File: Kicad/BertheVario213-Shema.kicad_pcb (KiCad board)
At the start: 2 copper layers, 8 parts

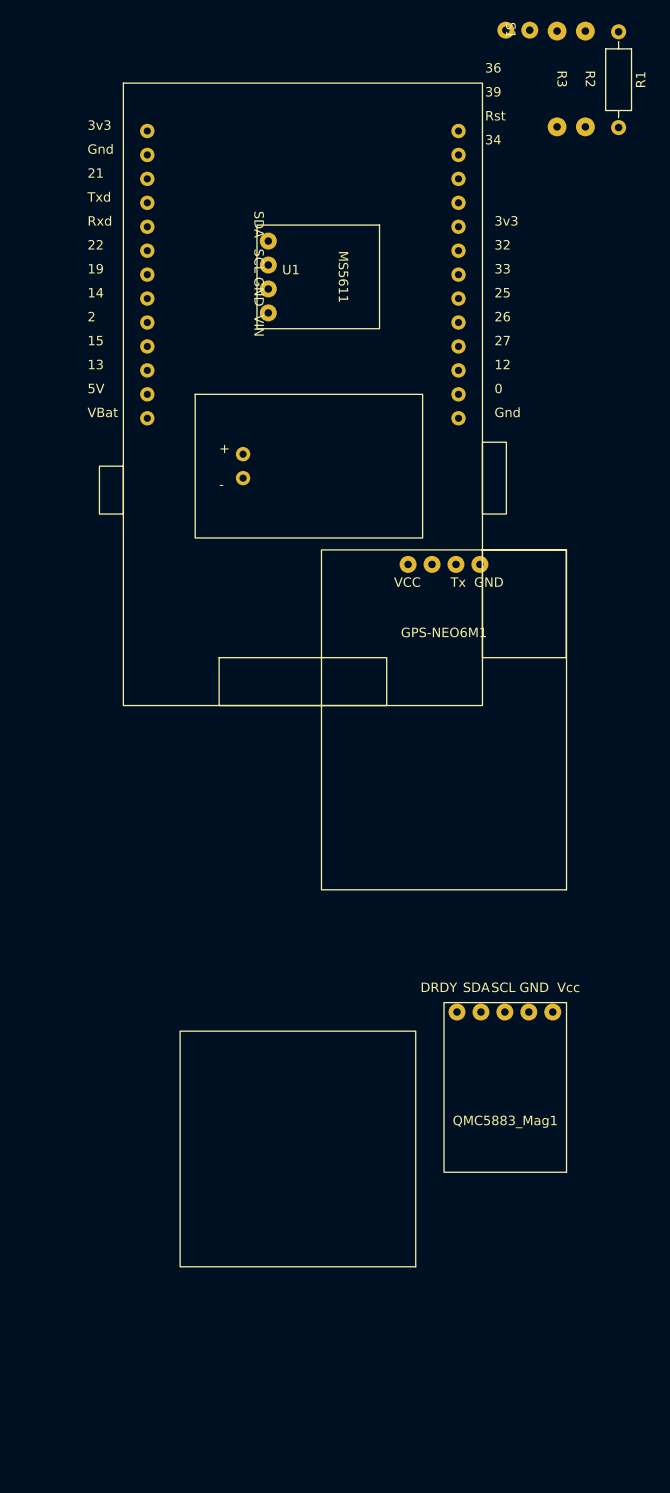
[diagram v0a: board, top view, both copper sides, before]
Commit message: progession pcb
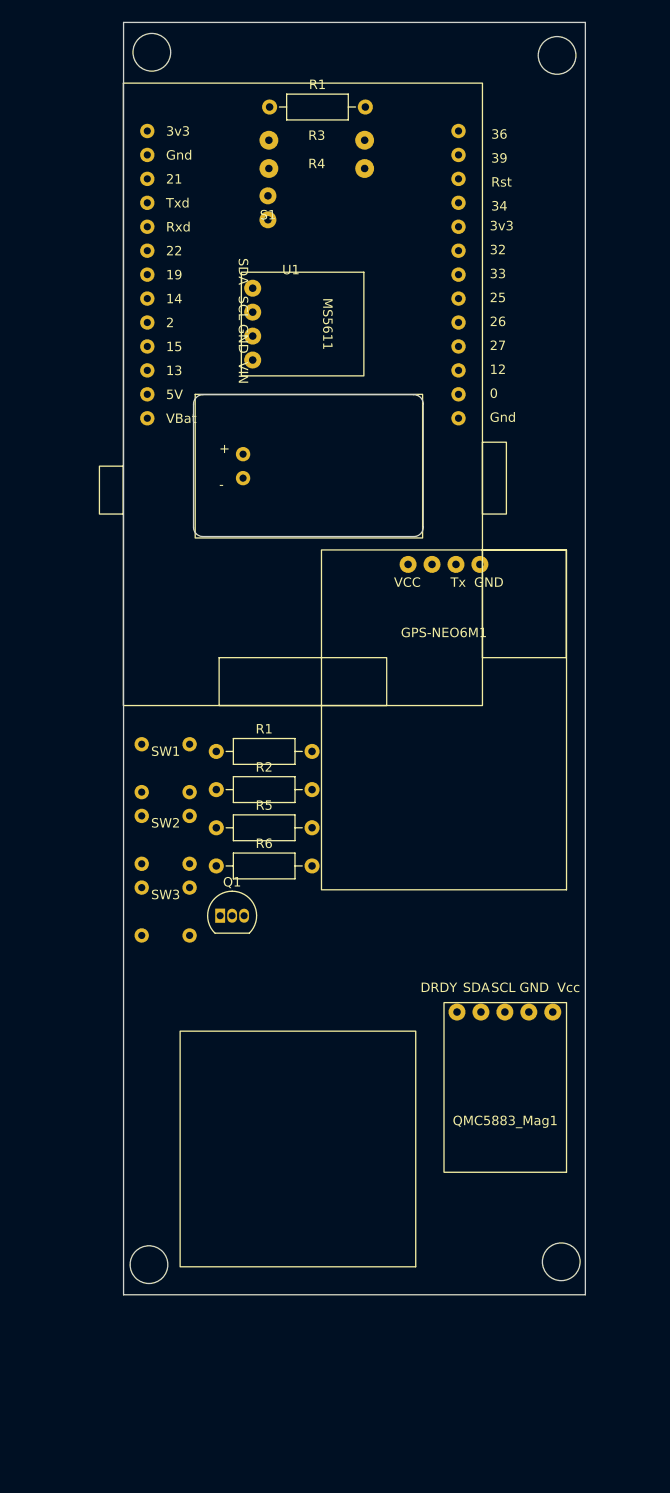
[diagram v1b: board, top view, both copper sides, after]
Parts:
- added Q1: S8050, Package_TO_SOT_THT:TO-92_Inline, F.Cu at (141.2, 117.3)
- added R1: 1K, Resistor_THT:R_Axial_DIN0207_L6.3mm_D2.5mm_P10.16mm_Horizontal, F.Cu at (140.8, 99.8)
- added R2: 10k, Resistor_THT:R_Axial_DIN0207_L6.3mm_D2.5mm_P10.16mm_Horizontal, F.Cu at (140.8, 103.9)
- added R5: 10K, Resistor_THT:R_Axial_DIN0207_L6.3mm_D2.5mm_P10.16mm_Horizontal, F.Cu at (140.8, 108.0)
- added R6: 10k, Resistor_THT:R_Axial_DIN0207_L6.3mm_D2.5mm_P10.16mm_Horizontal, F.Cu at (140.8, 112.0)
- added SW1: Gauche, BertheShema:switch, F.Cu at (135.5, 100.4)
- added SW2: Centre, BertheShema:switch, F.Cu at (135.5, 108.0)
- added SW3: Droit, BertheShema:switch, F.Cu at (135.5, 115.6)
- moved R1 37.9 mm to (146.5, 31.5), turned to 0 degrees
- moved S1 32.3 mm to (146.3, 43.4), turned to 0 degrees
- moved R3 29.2 mm to (151.5, 35.0), turned to 0 degrees
- moved R4 27.2 mm to (151.5, 38.0), turned to 0 degrees
- moved MS5611 5.27 mm to (147.1, 54.5)
- renumbered R2 to R3, R3 to R4
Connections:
- S1 pad 1: GNDREF -> Net-(Q1-C)
- S1 pad 2: Net-(R1-Pad1) -> Net-(U1-Vbat)
- U1 pad 13: (no net) -> Net-(U1-Bouton_Droit)
- U1 pad 14: (no net) -> Net-(U1-Bouton_Gauche)
- U1 pad 15: (no net) -> Net-(U1-Bouton_Centre)
- U1 pad 34: (no net) -> Net-(U1-Speaker)
- U1 pad 36: (no net) -> Net-(U1-VBat)
- U1 pad 6: unconnected-(U1-Vbat-Pad6) -> Net-(U1-Vbat)
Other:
- board outline added: 49 x 135 mm

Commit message: modif pcb
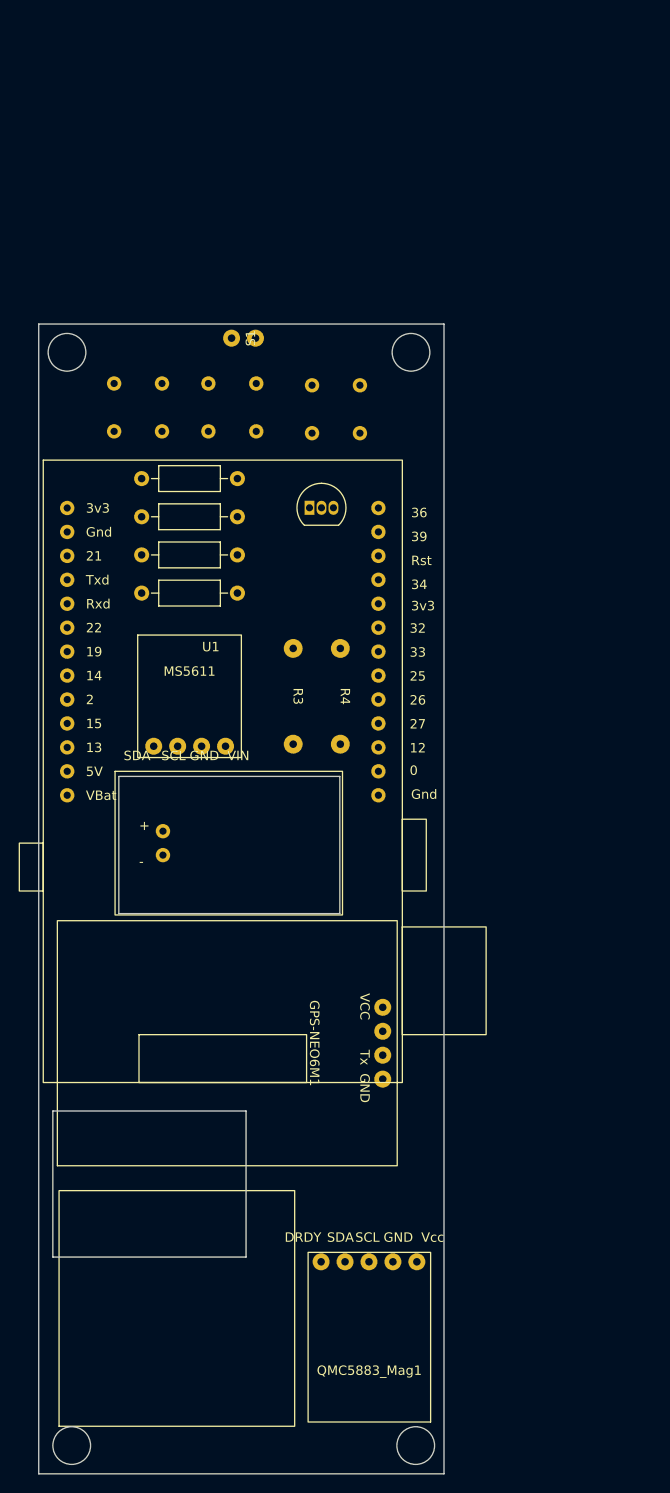
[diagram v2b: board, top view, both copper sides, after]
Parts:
- removed the R1 at (146.5, 31.5)
- S1: value Speaker 2W 8ohms -> Speaker 1W 80 ohms
- moved R3 59.1 mm to (149.0, 94.0), turned to -90 degrees
- moved R4 56.1 mm to (154.0, 94.0), turned to -90 degrees
- moved SW3 53.6 mm to (132.5, 62.1)
- moved GPS-NEO6M1 49.9 mm to (157.0, 130.8), turned to 90 degrees
- moved SW2 46.4 mm to (142.5, 62.1)
- moved Q1 44.3 mm to (150.7, 74.0)
- moved MS5611 43.4 mm to (138.0, 96.9), turned to 0 degrees
- moved SW1 42.2 mm to (153.5, 62.3)
- moved U1 40.9 mm to (140.3, 89.3)
- moved QMC5883_Mag1 30.2 mm to (157.1, 160.0)
- moved R2 30.0 mm to (132.9, 75.0)
- moved R5 30.0 mm to (132.9, 79.0)
- moved R6 30.0 mm to (132.9, 83.0)
- moved R1 30.0 mm to (132.9, 70.9)
- moved S1 12.6 mm to (145.0, 56.0), turned to 90 degrees
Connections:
- S1 pad 2: Net-(U1-Vbat) -> Net-(U1-5V)
- U1 pad 25: (no net) -> Net-(U1-Speaker)
- U1 pad 34: Net-(U1-Speaker) -> (no net)
- U1 pad 5: (no net) -> Net-(U1-5V)
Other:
- board size 49 x 135 mm -> 43 x 122 mm

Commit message: modif pcb
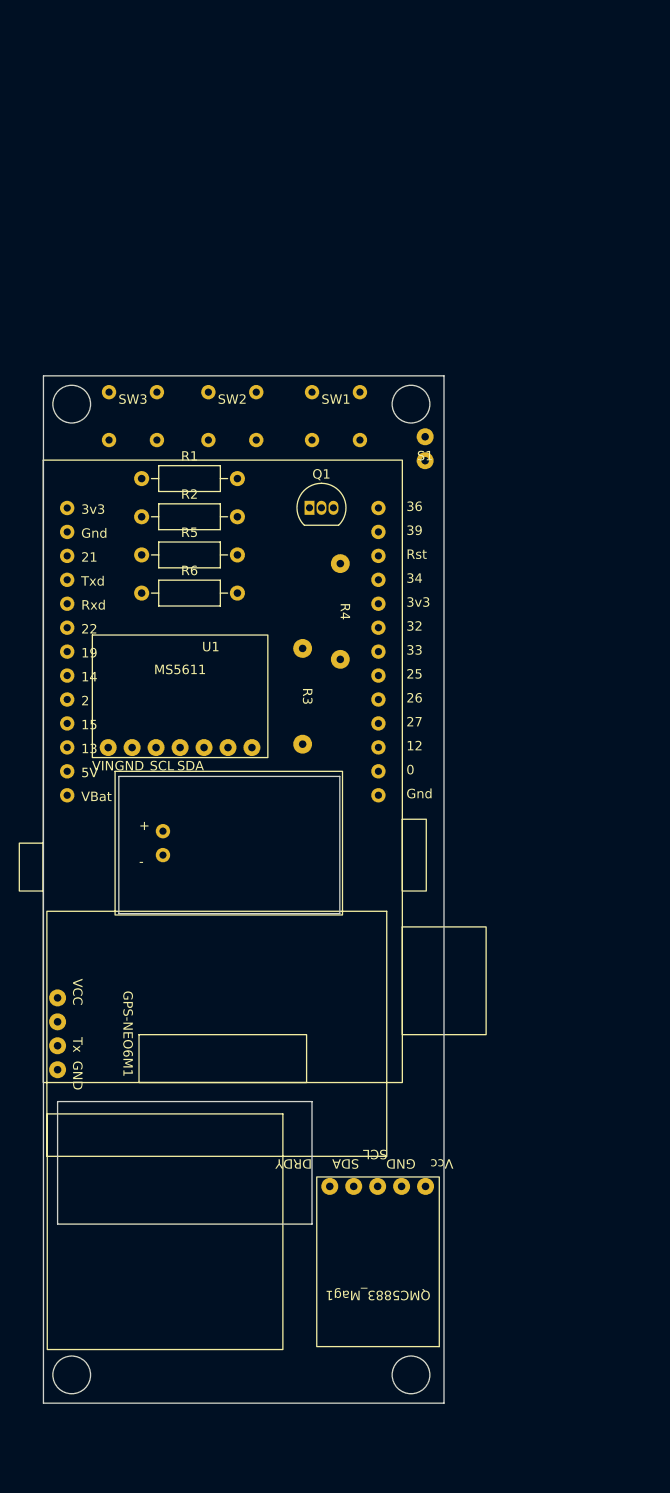
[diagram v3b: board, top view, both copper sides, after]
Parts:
- moved GPS-NEO6M1 31.1 mm to (125.9, 129.8), turned to -90 degrees
- moved S1 22.2 mm to (163.0, 69.0), turned to 0 degrees
- moved R4 9.00 mm to (154.0, 85.0)
- moved QMC5883_Mag1 8.05 mm to (158.0, 152.0)
- moved MS5611 4.81 mm to (133.2, 96.9)
- moved SW3 1.07 mm to (132.0, 63.0)
- moved R3 1.00 mm to (150.0, 94.0)
- moved SW2 0.92 mm to (142.5, 63.0)
- moved SW1 0.73 mm to (153.5, 63.0)
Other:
- board size 43 x 122 mm -> 42.5 x 109 mm
